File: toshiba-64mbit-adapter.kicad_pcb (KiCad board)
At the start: 2 copper layers, 9 parts, among them U1 TC5364205, U2 W29GL064C, U3 74HCT244, U4 74HCT244, U5 74HCT244, U6 74HCT244, U7 74HCT244, U8 TPS73633DBV

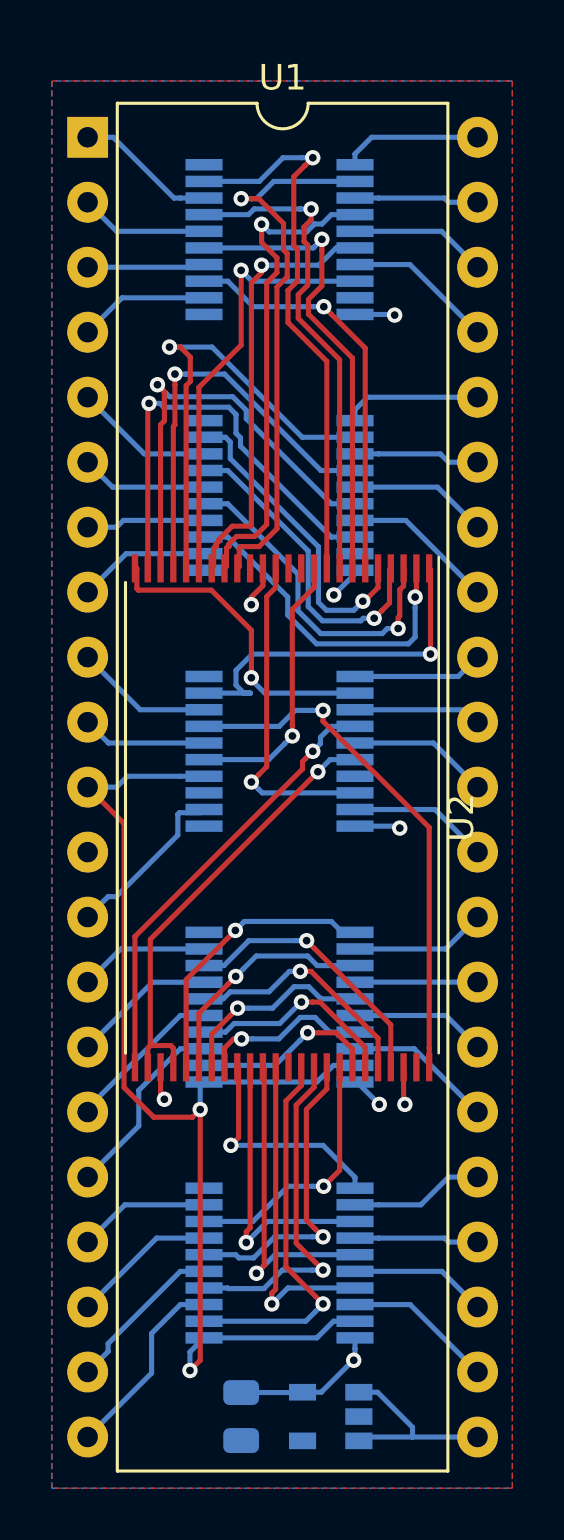
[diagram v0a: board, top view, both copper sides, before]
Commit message: v1.1
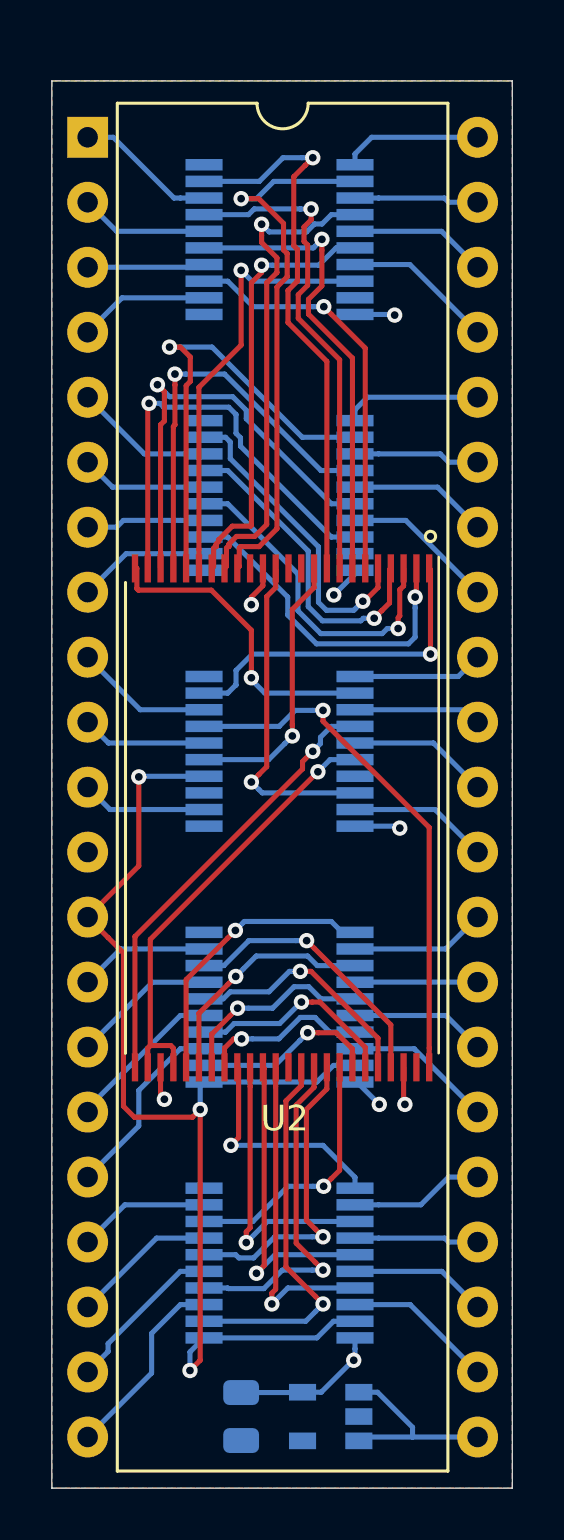
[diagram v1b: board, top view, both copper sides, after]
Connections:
- U1 pad 11: /E -> /A21
- U1 pad 13: /A21 -> /E
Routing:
- net /A21: track 6.77 -> 4.91 mm
- net /ma15: track 14.3 -> 13.2 mm
- net /E: track 46.0 -> 45.5 mm, vias 2 -> 3
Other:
- board outline added: 18 x 55 mm
- rule solder_mask_min_width: 0.25 -> 0.05
- board text added: "CC0 v1.1 2019"
- board text added: "github.com/tdaede/toshiba-64mbit-adapter"
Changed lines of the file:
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@@
   (general
     (thickness 1.6)
-    (drawings 0)
-    (tracks 578)
+    (drawings 7)
+    (tracks 573)
     (zones 0)
     (modules 9)
@@
     (pad_drill 0.762)
     (pad_to_mask_clearance 0)
-    (solder_mask_min_width 0.25)
+    (solder_mask_min_width 0.05)
     (aux_axis_origin 0 0)
     (visible_elements FFFFFF7F)
@@
     (tags "TSOP I 32")
     (attr smd)
-    (fp_text reference U2 (at 0 -7 270) (layer F.SilkS)
+    (fp_text reference U2 (at 11.75 -0.1) (layer F.SilkS)
       (effects (font (size 1 1) (thickness 0.15)))
     )
@@
     (tags capacitor)
     (attr smd)
-    (fp_text reference C1 (at 0 1.65 90) (layer B.SilkS)
+    (fp_text reference C1 (at 0 -1.7 90) (layer B.SilkS)
       (effects (font (size 1 1) (thickness 0.15)) (justify mirror))
     )
@@
     (tags SOT-23-5)
     (attr smd)
-    (fp_text reference U8 (at 0 2.9 180) (layer B.SilkS)
-      (effects (font (size 1 1) (thickness 0.15)) (justify mirror))
-    )
-    (fp_text value TPS73633DBV (at 0 -2.9 180) (layer B.Fab)
+    (fp_text reference U8 (at -2.7 0 270) (layer B.SilkS)
+      (effects (font (size 1 1) (thickness 0.15)) (justify mirror))
+    )
+    (fp_text value TPS73633DBV (at 1.45 -1.25 180) (layer B.Fab)
       (effects (font (size 1 1) (thickness 0.15)) (justify mirror))
     )
@@
     (descr "42-lead though-hole mounted DIP package, row spacing 15.24 mm (600 mils)")
     (tags "THT DIP DIL PDIP 2.54mm 15.24mm 600mil")
-    (fp_text reference U1 (at 7.62 -2.33) (layer F.SilkS)
+    (fp_text reference U1 (at 7.7 0.85) (layer F.SilkS) hide
       (effects (font (size 1 1) (thickness 0.15)))
     )
-    (fp_text value TC5364205 (at 7.62 53.13) (layer F.Fab)
+    (fp_text value TC5364205 (at 7.75 49.55) (layer F.Fab)
       (effects (font (size 1 1) (thickness 0.15)))
     )
@@
       (net 17 /A15))
     (pad 13 thru_hole oval (at 0 30.48) (size 1.6 1.6) (drill 0.8) (layers *.Cu *.Mask)
-      (net 18 /A21))
+      (net 22 /E))
     (pad 33 thru_hole oval (at 15.24 22.86) (size 1.6 1.6) (drill 0.8) (layers *.Cu *.Mask)
       (net 19 /A16))
@@
       (net 21 /A20))
     (pad 11 thru_hole oval (at 0 25.4) (size 1.6 1.6) (drill 0.8) (layers *.Cu *.Mask)
-      (net 22 /E))
+      (net 18 /A21))
     (pad 31 thru_hole oval (at 15.24 27.94) (size 1.6 1.6) (drill 0.8) (layers *.Cu *.Mask)
       (net 20 GND))
@@
       (net 41 /A18))
   )
+  (gr_circle (center 124.4 76.6) (end 124.6 76.6) (layer F.SilkS) (width 0.12))
+  (gr_text "CC0 v1.1 2019" (at 113.3 87.05 270) (layer B.SilkS)
+    (effects (font (size 1 1) (thickness 0.15)) (justify mirror))
+  )
+  (gr_text github.com/tdaede/toshiba-64mbit-adapter (at 124.1 87.25 270) (layer B.SilkS)
+    (effects (font (size 1 1) (thickness 0.15)) (justify mirror))
+  )
+  (gr_line (start 109.6 113.8) (end 109.6 58.8) (layer Edge.Cuts) (width 0.05))
+  (gr_line (start 127.6 113.8) (end 109.6 113.8) (layer Edge.Cuts) (width 0.05))
+  (gr_line (start 127.6 58.8) (end 127.6 113.8) (layer Edge.Cuts) (width 0.05))
+  (gr_line (start 109.6 58.8) (end 127.6 58.8) (layer Edge.Cuts) (width 0.05))
   (segment (start 122.1 61) (end 121.45 61.65) (width 0.2) (layer B.Cu) (net 1))
   (segment (start 121.45 61.65) (end 121.45 62.075) (width 0.2) (layer B.Cu) (net 1))
@@
   (segment (start 125.485 82.075) (end 126.24 81.32) (width 0.2) (layer B.Cu) (net 17))
   (segment (start 121.45 82.075) (end 125.485 82.075) (width 0.2) (layer B.Cu) (net 17))
-  (segment (start 115.525 87.275) (end 115.55 87.275) (width 0.2) (layer B.Cu) (net 18))
-  (segment (start 115.400001 87.399999) (end 115.525 87.275) (width 0.2) (layer B.Cu) (net 18))
-  (segment (start 111.799999 90.680001) (end 112.119999 90.680001) (width 0.2) (layer B.Cu) (net 18))
-  (segment (start 111 91.48) (end 111.799999 90.680001) (width 0.2) (layer B.Cu) (net 18))
-  (segment (start 114.524999 88.275001) (end 114.524999 87.459999) (width 0.2) (layer B.Cu) (net 18))
-  (segment (start 114.584999 87.399999) (end 115.400001 87.399999) (width 0.2) (layer B.Cu) (net 18))
-  (segment (start 114.524999 87.459999) (end 114.584999 87.399999) (width 0.2) (layer B.Cu) (net 18))
-  (segment (start 112.119999 90.680001) (end 114.524999 88.275001) (width 0.2) (layer B.Cu) (net 18))
+  (segment (start 111.875 87.275) (end 115.55 87.275) (width 0.2) (layer B.Cu) (net 18))
+  (segment (start 111 86.4) (end 111.875 87.275) (width 0.2) (layer B.Cu) (net 18))
   (segment (start 125.755 83.375) (end 126.24 83.86) (width 0.2) (layer B.Cu) (net 19))
   (segment (start 121.45 83.375) (end 125.755 83.375) (width 0.2) (layer B.Cu) (net 19))
@@
   (segment (start 124.515 84.675) (end 126.24 86.4) (width 0.2) (layer B.Cu) (net 21))
   (segment (start 121.45 84.675) (end 124.515 84.675) (width 0.2) (layer B.Cu) (net 21))
-  (segment (start 114.625 85.975) (end 115.55 85.975) (width 0.2) (layer B.Cu) (net 22))
-  (segment (start 112.55637 85.975) (end 114.625 85.975) (width 0.2) (layer B.Cu) (net 22))
-  (segment (start 112.13137 86.4) (end 112.55637 85.975) (width 0.2) (layer B.Cu) (net 22))
-  (segment (start 111 86.4) (end 112.13137 86.4) (width 0.2) (layer B.Cu) (net 22))
   (segment (start 120.609998 97.275) (end 121.45 97.275) (width 0.2) (layer B.Cu) (net 22))
   (segment (start 119.959998 97.925) (end 120.609998 97.275) (width 0.2) (layer B.Cu) (net 22))
@@
   (segment (start 115 108.475) (end 115.55 107.925) (width 0.2) (layer B.Cu) (net 22))
   (segment (start 115 109.2) (end 115 108.475) (width 0.2) (layer B.Cu) (net 22))
-  (segment (start 112.424999 98.140001) (end 113.584997 99.299999) (width 0.2) (layer F.Cu) (net 22))
-  (segment (start 115.100001 99.299999) (end 115.4 99) (width 0.2) (layer F.Cu) (net 22))
-  (segment (start 113.584997 99.299999) (end 115.100001 99.299999) (width 0.2) (layer F.Cu) (net 22))
-  (segment (start 111 86.4) (end 112.424999 87.824999) (width 0.2) (layer F.Cu) (net 22))
-  (segment (start 112.424999 87.824999) (end 112.424999 98.140001) (width 0.2) (layer F.Cu) (net 22))
+  (via (at 113 86) (size 0.6) (drill 0.3) (layers F.Cu B.Cu) (net 22))
+  (segment (start 115.55 85.975) (end 113.025 85.975) (width 0.2) (layer B.Cu) (net 22))
+  (segment (start 113.025 85.975) (end 113 86) (width 0.2) (layer B.Cu) (net 22))
+  (segment (start 113 89.48) (end 111 91.48) (width 0.2) (layer F.Cu) (net 22))
+  (segment (start 113 86) (end 113 89.48) (width 0.2) (layer F.Cu) (net 22))
+  (segment (start 112.4 92.88) (end 111.799999 92.279999) (width 0.2) (layer F.Cu) (net 22))
+  (segment (start 112.4 98.871998) (end 112.4 92.88) (width 0.2) (layer F.Cu) (net 22))
+  (segment (start 112.828001 99.299999) (end 112.4 98.871998) (width 0.2) (layer F.Cu) (net 22))
+  (segment (start 115.4 99) (end 115.100001 99.299999) (width 0.2) (layer F.Cu) (net 22))
+  (segment (start 111.799999 92.279999) (end 111 91.48) (width 0.2) (layer F.Cu) (net 22))
+  (segment (start 115.100001 99.299999) (end 112.828001 99.299999) (width 0.2) (layer F.Cu) (net 22))
   (segment (start 111.815 84.675) (end 115.55 84.675) (width 0.2) (layer B.Cu) (net 23))
   (segment (start 111 83.86) (end 111.815 84.675) (width 0.2) (layer B.Cu) (net 23))
@@
   (segment (start 116.799999 81.836989) (end 117.436988 81.2) (width 0.2) (layer B.Cu) (net 65))
   (segment (start 116.799999 82.412991) (end 116.799999 81.836989) (width 0.2) (layer B.Cu) (net 65))
-  (segment (start 117.111999 82.724991) (end 116.799999 82.412991) (width 0.2) (layer B.Cu) (net 65))
-  (segment (start 117.359302 82.725) (end 117.359293 82.724991) (width 0.2) (layer B.Cu) (net 65))
-  (segment (start 115.55 82.725) (end 117.359302 82.725) (width 0.2) (layer B.Cu) (net 65))
-  (segment (start 117.359293 82.724991) (end 117.111999 82.724991) (width 0.2) (layer B.Cu) (net 65))
   (segment (start 124.4 81.2) (end 124.4 77.9) (width 0.2) (layer F.Cu) (net 65))
   (segment (start 124.4 77.9) (end 124.35 77.85) (width 0.2) (layer F.Cu) (net 65))
+  (segment (start 116.787009 82.412991) (end 116.799999 82.412991) (width 0.2) (layer B.Cu) (net 65))
+  (segment (start 116.475 82.725) (end 116.787009 82.412991) (width 0.2) (layer B.Cu) (net 65))
+  (segment (start 115.55 82.725) (end 116.475 82.725) (width 0.2) (layer B.Cu) (net 65))
   (segment (start 113.35 77.85) (end 113.35 71.45) (width 0.2) (layer F.Cu) (net 66))
   (via (at 113.4 71.4) (size 0.6) (drill 0.3) (layers F.Cu B.Cu) (net 66))
